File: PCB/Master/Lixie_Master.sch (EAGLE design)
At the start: 9 parts, among them IC1 FT232RL, J1 65100516121, U1 ATTINY406-MFR

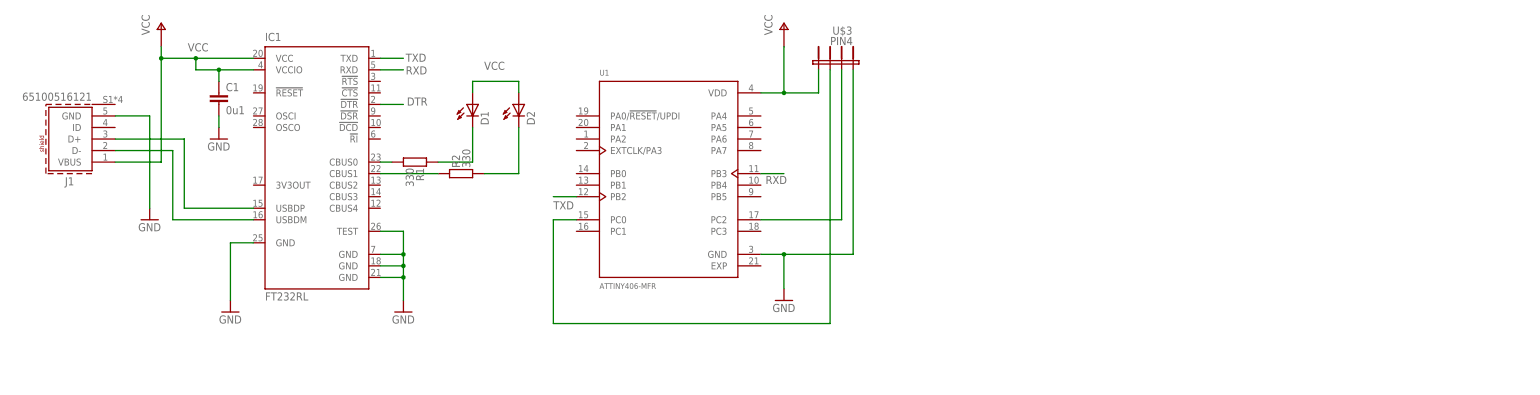
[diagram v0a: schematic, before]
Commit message: V04
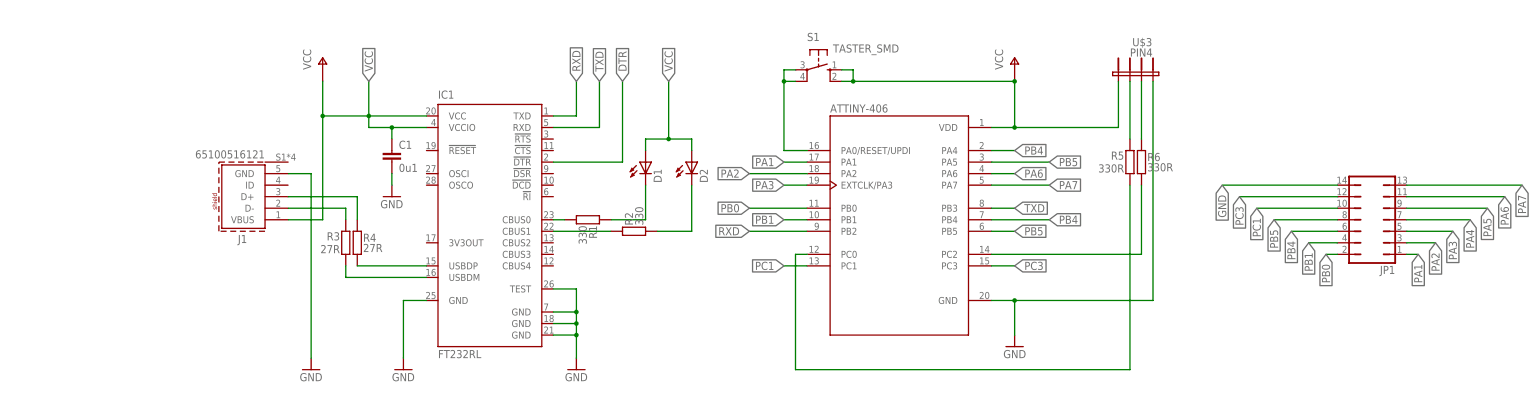
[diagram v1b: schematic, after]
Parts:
- removed U1: ATTINY406-MFR, ATTINY406-MFR:ATTINY406-MFR
- added ATTINY-406: (no value), SOIC127P1032X265-20N:ATTINY-406SN
- added JP1: (no value), jumper:JP7Q
- added R3, R4: 27R, 0_HTL_analog:R1206
- added R5, R6: 330R, 0_HTL_analog:R1206
- added S1: TASTER_SMD, 0_HTL_MegaCard_V3:TASTER_SMD
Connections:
- new net N$10: IC1.USBDP, R4.1
- new net N$11: ATTINY-406.PA0/RESET/UPDI, S1.P, S1.P1
- new net N$12: R5.2, U$3.2
- new net N$13: R6.2, U$3.3
- new net N$4: J1.D-, R3.2
- new net PA1: ATTINY-406.PA1, JP1.1
- new net PA2: ATTINY-406.PA2, JP1.3
- new net PA3: ATTINY-406.EXTCLK/PA3, JP1.5
- new net PA4: JP1.7
- new net PA5: JP1.9
- new net PA6: ATTINY-406.PA6, JP1.11
- new net PA7: ATTINY-406.PA7, JP1.13
- new net PB0: ATTINY-406.PB0, JP1.2
- new net PB1: ATTINY-406.PB1, JP1.4
- new net PB4: ATTINY-406.PA4, ATTINY-406.PB4, JP1.6
- new net PB5: ATTINY-406.PA5, ATTINY-406.PB5, JP1.8
- new net PC1: ATTINY-406.PC1, JP1.10
- new net PC3: ATTINY-406.PC3, JP1.12
- net GND: now also ATTINY-406.GND, JP1.14; no longer U1.GND
- net N$1: now also R4.2; no longer IC1.USBDP
- net N$2: now also R3.1; no longer J1.D-
- net N$8: now also ATTINY-406.PC0, R5.1; no longer U$3.2, U1.PC0
- net N$9: now also ATTINY-406.PC2, R6.1; no longer U$3.3, U1.PC2
- net RXD: now also ATTINY-406.PB2, IC1.TXD; no longer IC1.RXD, U1.PB3
- net TXD: now also ATTINY-406.PB3, IC1.RXD; no longer IC1.TXD, U1.PB2
- net VCC: now also ATTINY-406.VDD, S1.S, S1.S1; no longer U1.VDD
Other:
- moved on the sheet: C1, D1, D2, IC1, J1, R1, R2, U$3
